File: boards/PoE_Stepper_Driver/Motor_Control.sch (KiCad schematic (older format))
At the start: 22 parts, among them J2 Motor, SW1 STO_L, SW2 STO_R, U15 TMC429-I, U16 TMC2660C-PA

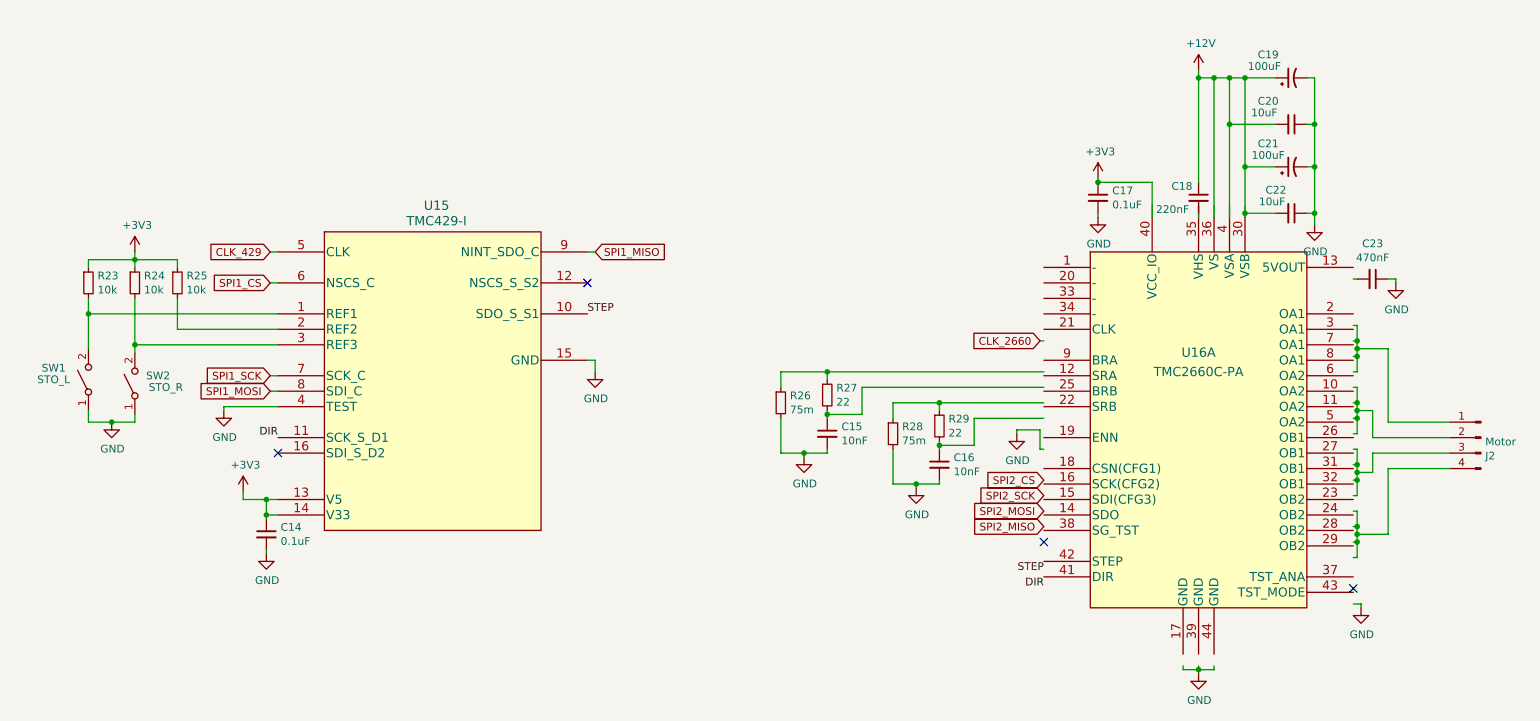
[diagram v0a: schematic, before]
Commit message: started board layout
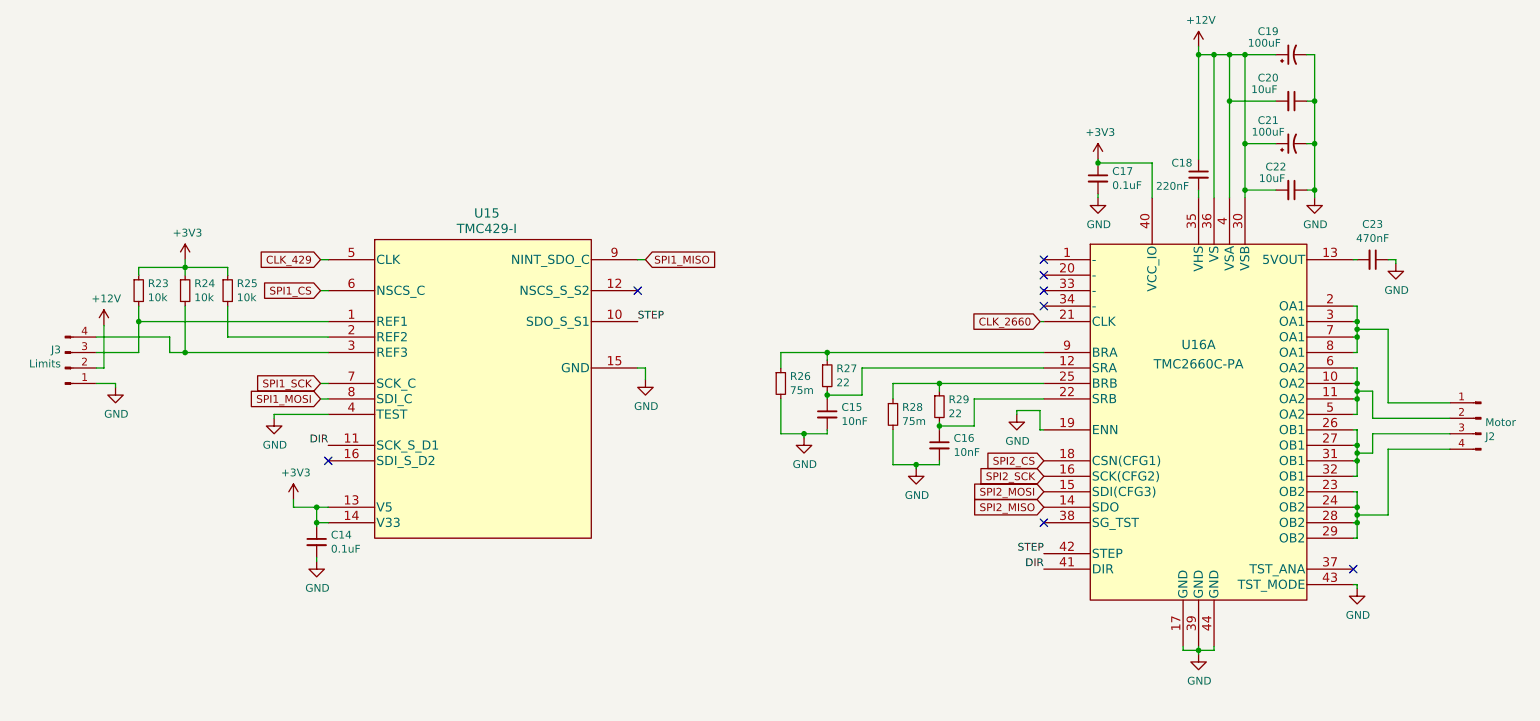
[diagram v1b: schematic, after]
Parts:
- removed SW1: STO_L, symbol Switch:SW_SPST
- removed SW2: STO_R, symbol Switch:SW_SPST
- added J3: Limits, symbol Connector:Conn_01x04_Male
- C14, C17: footprint (none) -> Capacitor_SMD:C_0805_2012Metric_Pad1.15x1.40mm_HandSolder
- J2: footprint (none) -> Connector_JST:JST_PH_B4B-PH-K_1x04_P2.00mm_Vertical
- U15: footprint SSOP16_150MIL_TRI -> Package_SO:SSOP-16_3.9x4.9mm_P0.635mm
- U16: footprint QFP_2660C-PA_TRI -> Package_QFP:PQFP-44_10x10mm_P0.8mm
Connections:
- wire segments 150 -> 153
- no-connect marks 4 -> 8
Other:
- moved on the sheet: C14, C15, C16, C17, C18, C19, C20, C21, C22, C23, J2, R23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
